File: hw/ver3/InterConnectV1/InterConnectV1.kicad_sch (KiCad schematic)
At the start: 3 parts, among them J3 RJ45, J4 Conn_02x04_Odd_Even, U5 SP3485EN

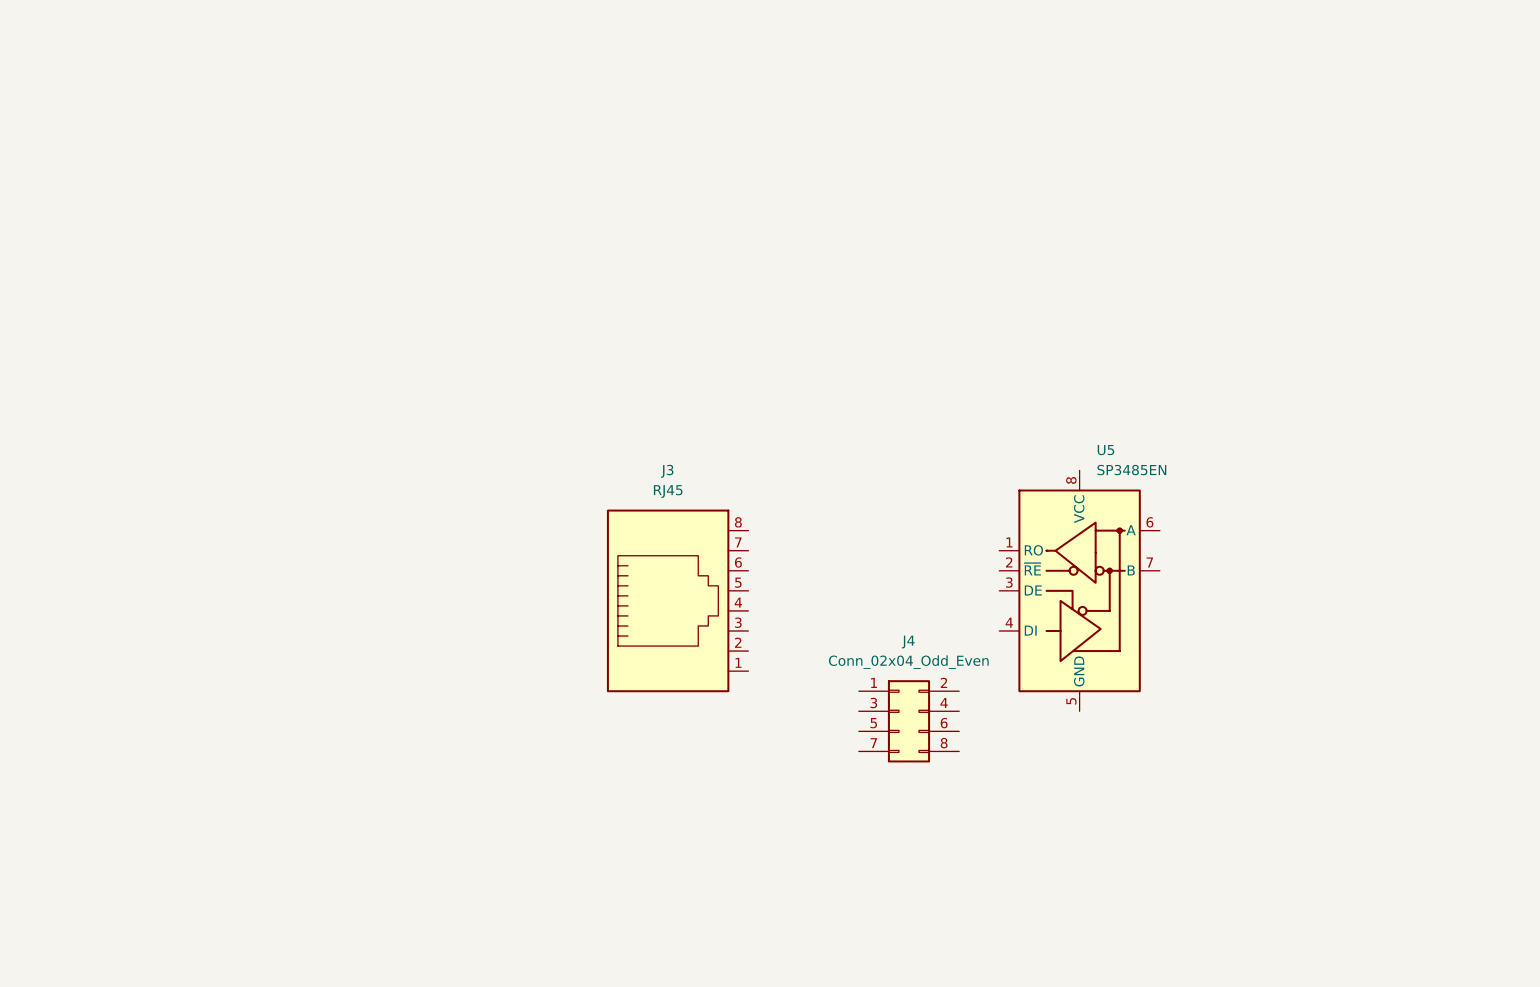
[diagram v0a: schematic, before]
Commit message: Initial schematic for InterConnectV1
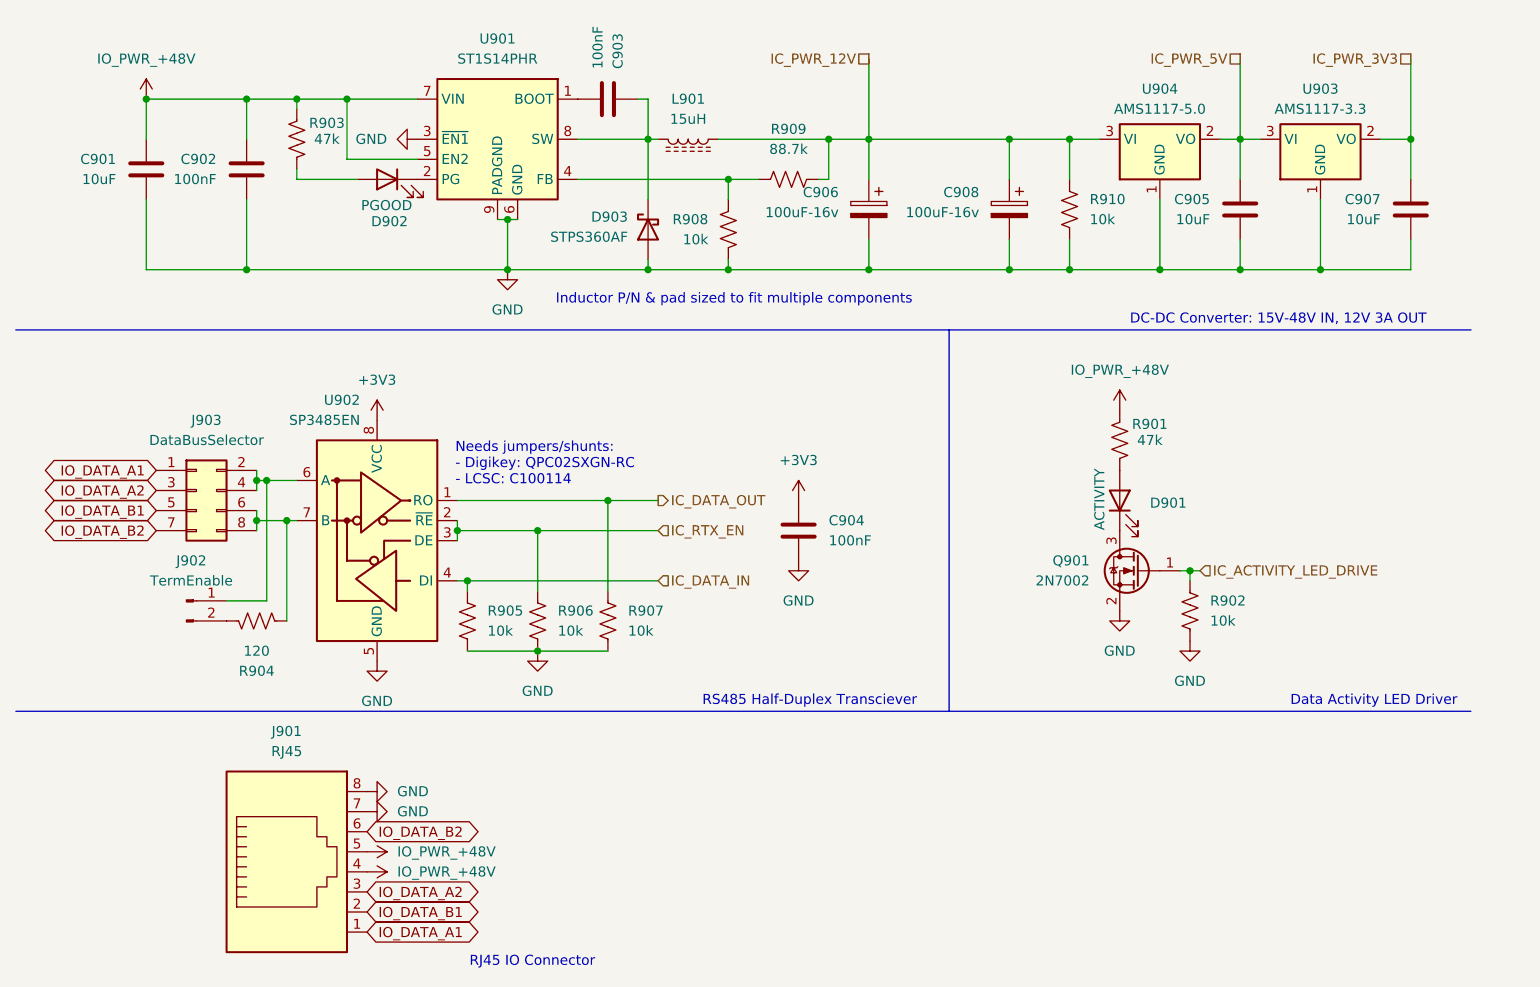
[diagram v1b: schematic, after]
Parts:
- added C901, C905, C907: 10uF, Capacitor_SMD:C_0603_1608Metric, symbol Device:C
- added C902, C903, C904: 100nF, Capacitor_SMD:C_0603_1608Metric, symbol Device:C
- added C906, C908: 100uF-16v, Capacitor_SMD:CP_Elec_6.3x5.4, symbol Device:C_Polarized
- added D901: ACTIVITY, LED_SMD:LED_0805_2012Metric, symbol Device:LED
- added D902: PGOOD, LED_SMD:LED_0805_2012Metric, symbol Device:LED
- added D903: STPS360AF, Diode_SMD:D_SOD-128, symbol Device:D_Schottky
- added J902: TermEnable, Connector_PinHeader_2.54mm:PinHeader_1x02_P2.54mm_Vertical, symbol Connector:Conn_01x02_Pin
- added L901: 15uH, Inductor_SMD:L_12x12mm_H4.5mm, symbol Device:L_Ferrite
- added Q901: 2N7002, Package_TO_SOT_SMD:SOT-23, symbol Transistor_FET:2N7002
- added R901, R903: 47k, Resistor_SMD:R_0603_1608Metric, symbol Device:R_US
- added R902, R905, R906, R907, R908, R910: 10k, Resistor_SMD:R_0603_1608Metric, symbol Device:R_US
- added R904: 120, Resistor_SMD:R_0603_1608Metric, symbol Device:R_US
- added R909: 88.7k, Resistor_SMD:R_0603_1608Metric, symbol Device:R_US
- added U901: ST1S14PHR, Package_SO:TI_SO-PowerPAD-8, symbol Regulator_Switching:ST1S14PHR
- added U903: AMS1117-3.3, Package_TO_SOT_SMD:SOT-223-3_TabPin2, symbol Regulator_Linear:AMS1117-3.3
- added U904: AMS1117-5.0, Package_TO_SOT_SMD:SOT-223-3_TabPin2, symbol Regulator_Linear:AMS1117-5.0
- J901: renamed from J3; footprint (none) -> Connector_RJ:RJ45_Amphenol_54602-x08_Horizontal; Digikey (none) -> 609-1046-ND; LCSC (none) -> C2847314
- J903: renamed from J4; value Conn_02x04_Odd_Even -> DataBusSelector; Digikey (none) -> PH2-08-UA; LCSC (none) -> C492421
- U902: renamed from U5; Digikey (none) -> 4518-SP3485EENTR-ND; LCSC (none) -> C668205
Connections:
- net IO_DATA_A1: now reaches J903.1 (Pin_1)
- net IO_DATA_A1: now also J901.1
- net at J903.2 (Pin_2): now also J903.4 (Pin_4), U902.6 (A), J902.1 (Pin_1)
- net IO_DATA_A2: now reaches J903.3 (Pin_3)
- net IO_DATA_A2: now also J901.3
- net IO_DATA_B1: now reaches J903.5 (Pin_5)
- net IO_DATA_B1: now also J901.2
- net at J903.6 (Pin_6): now also J903.8 (Pin_8), U902.7 (B), R904.1
- net IO_DATA_B2: now reaches J903.7 (Pin_7)
- net IO_DATA_B2: now also J901.6
- net IO_PWR_+48V: now reaches J901.4
- net IO_PWR_+48V: now also J901.5, C901.1, C902.1, R901.1, R903.1, U901.5 (EN2), U901.7 (VIN)
- net GND: now reaches J901.7
- net GND: now also J901.8, U902.5 (GND), C901.2, C902.2, C904.2, C905.2, C906.2, C907.2, C908.2, D903.2 (A), Q901.2 (S), R902.1, R905.1, R906.1, R907.1, R908.1, R910.1, U901.3 (~{EN1}), U901.6 (GND), U901.9 (PADGND), U903.1 (GND), U904.1 (GND)
- net IC_DATA_OUT: now reaches U902.1 (RO)
- net IC_DATA_OUT: now also R907.2
- net IC_RTX_EN: now reaches U902.2 (~{RE})
- net IC_RTX_EN: now also U902.3 (DE), R906.2
- net IC_DATA_IN: now reaches U902.4 (DI)
- net IC_DATA_IN: now also R905.2
- net +3V3: now reaches U902.8 (VCC)
- net +3V3: now also C904.1
- new net: C903.1, D903.1 (K), L901.2, U901.8 (SW)
- new net: D901.2 (A), R901.2
- new net: D902.1 (K), U901.2 (PG)
- new net: D902.2 (A), R903.2
- new net: R908.2, R909.2, U901.4 (FB)
- new net: C903.2, U901.1 (BOOT)
- new net: J902.2 (Pin_2), R904.2
- new net: D901.1 (K), Q901.3 (D)
- new net IC_ACTIVITY_LED_DRIVE: Q901.1 (G), R902.2
- new net IC_PWR_12V: C906.1, C908.1, L901.1, R909.1, R910.2, U904.3 (VI)
- new net IC_PWR_3V3: C907.1, U903.2 (VO)
- new net IC_PWR_5V: C905.1, U903.3 (VI), U904.2 (VO)
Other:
- note added: "DC-DC Converter: 15V-48V IN, 12V 3A OUT"
- note added: "Data Activity LED Driver"
- note added: "Inductor P/N & pad sized to fit multiple components"
- note added: "Needs jumpers/shunts: - Digikey: QPC02SXGN-RC - LCSC: C100114"
- note added: "RJ45 IO Connector"
- note added: "RS485 Half-Duplex Transciever"
- moved on the sheet: J901, J903, U902
